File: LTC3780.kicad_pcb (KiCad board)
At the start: 2 copper layers, 100 x 60 mm, 62 parts, among them J1 Screw_Terminal_01x02, J2 Screw_Terminal_01x02, Q2 IPD100N04S402ATMA1, Q3 IPD100N04S402ATMA1, Q4 IPD100N04S402ATMA1, Q5 IPD100N04S402ATMA1, U1 LTC3780EGPBF

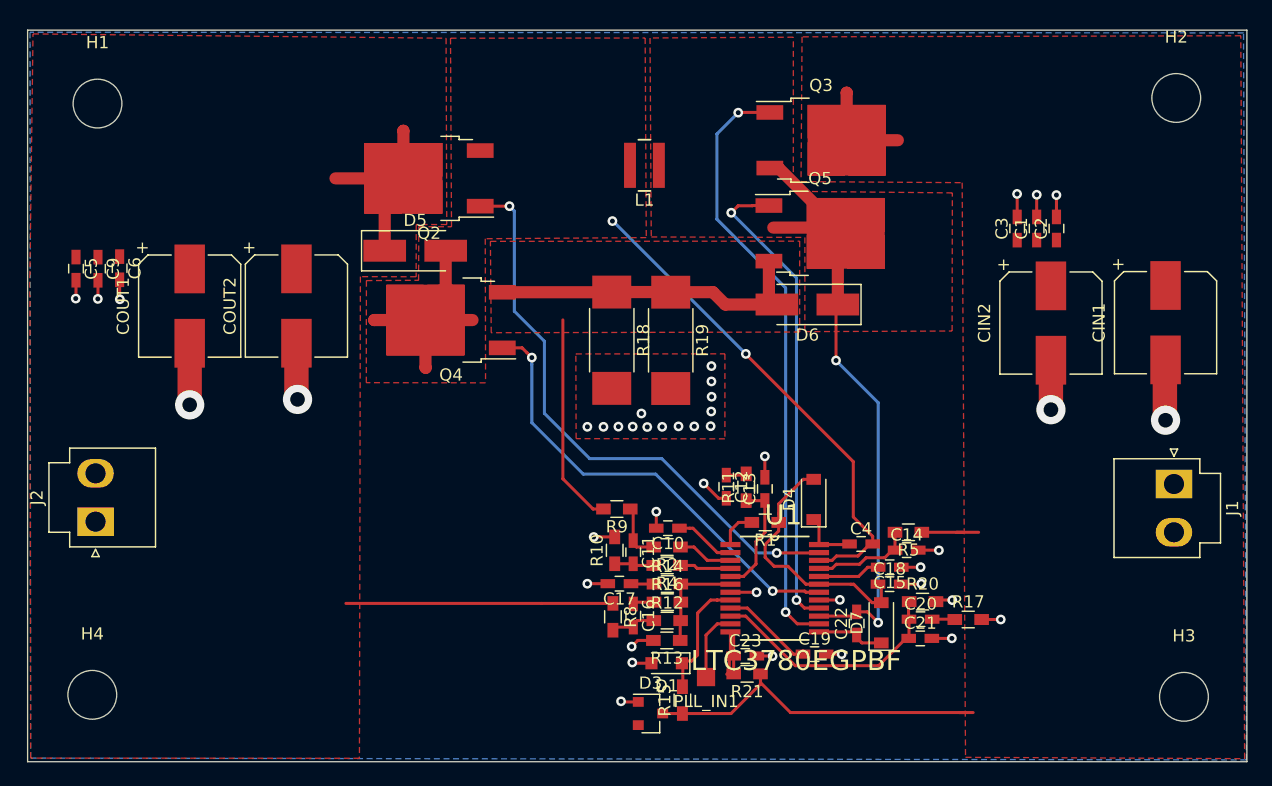
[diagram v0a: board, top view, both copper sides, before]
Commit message: Updating to latest version tidied routing
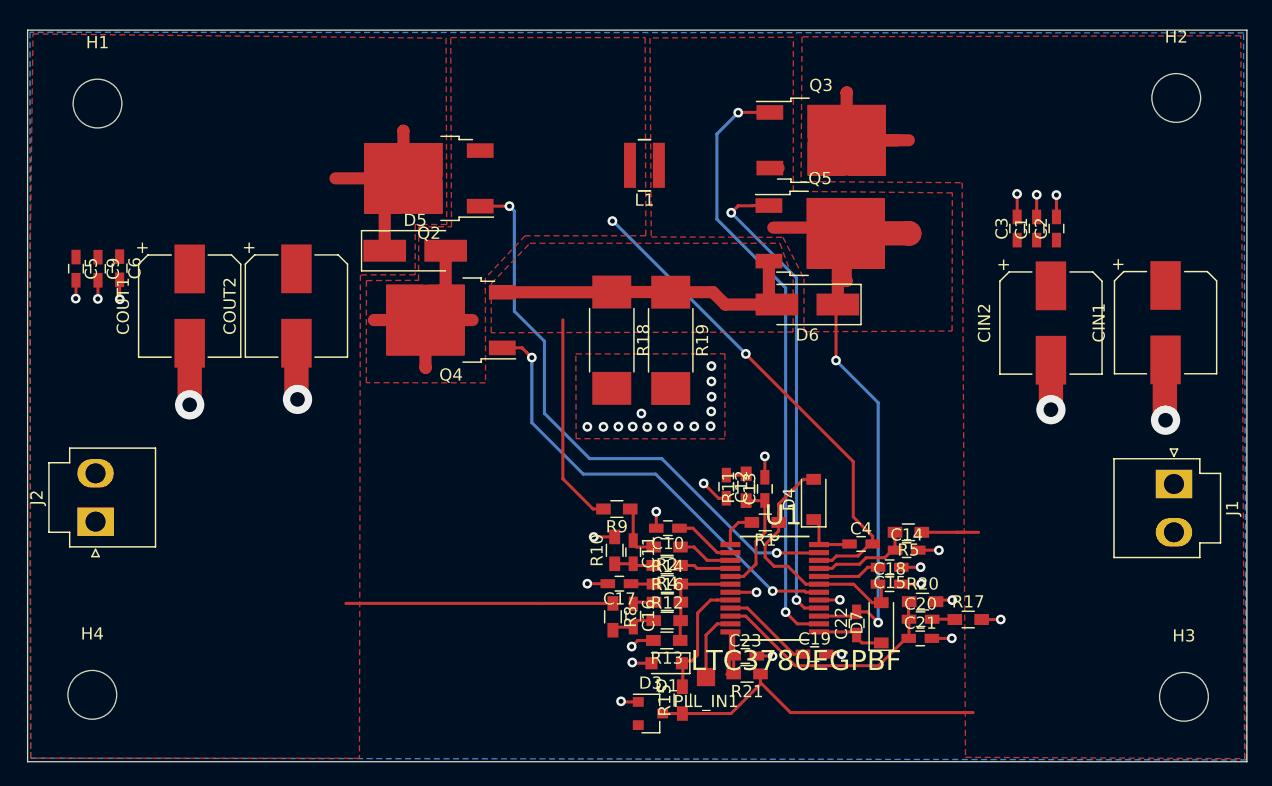
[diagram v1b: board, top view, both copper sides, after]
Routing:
- net +VSW: track 42.7 -> 47.9 mm
- net SW2: track 63.5 -> 60.4 mm
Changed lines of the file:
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@@
     (thickness 1.6)
     (drawings 6)
-    (tracks 348)
+    (tracks 355)
     (zones 0)
     (modules 62)
@@
   (segment (start 180.56606 102.98176) (end 194.41668 102.98176) (width 0.25) (layer F.Cu) (net 1))
   (segment (start 194.41668 102.98176) (end 194.88912 102.98176) (width 0.25) (layer F.Cu) (net 1))
+  (segment (start 185.17304 56.0451) (end 190.27648 56.0451) (width 1) (layer F.Cu) (net 1))
+  (segment (start 185.17304 52.1451) (end 185.2041 52.11404) (width 1) (layer F.Cu) (net 1))
   (via (at 211.328 79.0067) (size 2.4) (drill 1.2) (layers F.Cu B.Cu) (net 2))
   (segment (start 211.27466 79.0829) (end 211.27466 74.55608) (width 2) (layer F.Cu) (net 2) (status 10))
@@
   (segment (start 184.3024 74.10704) (end 184.3024 69.66712) (width 0.25) (layer F.Cu) (net 21) (status 20))
   (segment (start 184.45226 66.23518) (end 183.42242 65.20534) (width 0.25) (layer F.Cu) (net 21) (status 30))
-  (segment (start 179.44218 58.3251) (end 184.79742 63.68034) (width 0.25) (layer F.Cu) (net 21) (status 30))
   (segment (start 184.79742 63.68034) (end 185.09742 63.68034) (width 0.25) (layer F.Cu) (net 21) (status 30))
   (segment (start 178.87304 58.3251) (end 179.44218 58.3251) (width 0.25) (layer F.Cu) (net 21) (status 30))
   (segment (start 184.45226 64.3255) (end 185.09742 63.68034) (width 2.5) (layer F.Cu) (net 21))
-  (segment (start 179.59218 58.3251) (end 183.42242 62.15534) (width 1) (layer F.Cu) (net 21))
   (segment (start 178.87304 58.3251) (end 179.59218 58.3251) (width 1) (layer F.Cu) (net 21))
   (segment (start 184.45226 63.18518) (end 183.42242 62.15534) (width 1) (layer F.Cu) (net 21))
-  (segment (start 184.45226 69.51726) (end 184.45226 63.18518) (width 1) (layer F.Cu) (net 21))
   (segment (start 184.79742 63.68034) (end 184.32752 63.21044) (width 1) (layer F.Cu) (net 21))
   (segment (start 184.32752 63.21044) (end 179.15636 63.21044) (width 1) (layer F.Cu) (net 21))
+  (segment (start 190.29742 63.68034) (end 190.32028 63.7032) (width 2) (layer F.Cu) (net 21))
+  (segment (start 185.09742 63.68034) (end 190.29742 63.68034) (width 2) (layer F.Cu) (net 21))
+  (segment (start 184.45226 67.54622) (end 184.45226 63.18518) (width 1) (layer F.Cu) (net 21))
+  (segment (start 184.45226 69.51726) (end 184.45226 67.54622) (width 1) (layer F.Cu) (net 21))
+  (segment (start 185.16854 67.5767) (end 184.48274 67.5767) (width 1) (layer F.Cu) (net 21))
+  (segment (start 185.09742 67.50558) (end 185.16854 67.5767) (width 1) (layer F.Cu) (net 21))
+  (segment (start 184.48274 67.5767) (end 184.45226 67.54622) (width 1) (layer F.Cu) (net 21))
+  (segment (start 185.09742 63.68034) (end 185.09742 67.50558) (width 1) (layer F.Cu) (net 21))
   (segment (start 175.641 98.20652) (end 175.54952 98.298) (width 0.25) (layer F.Cu) (net 22) (status 30))
   (segment (start 175.641 96.3676) (end 175.641 98.20652) (width 0.25) (layer F.Cu) (net 22) (status 30))
@@
     (polygon
       (pts
-        (xy 180.80228 47.59452) (xy 169.04716 47.65802) (xy 169.14876 63.97752) (xy 181.7497 64.01308) (xy 181.74462 71.7423)
-        (xy 193.82232 71.6915) (xy 193.84264 60.3631) (xy 180.7972 60.23356)
+        (xy 180.80228 47.59452) (xy 169.04716 47.65802) (xy 169.14876 63.97752) (xy 179.95392 64.008) (xy 181.67604 67.39382)
+        (xy 181.67858 71.75246) (xy 193.82232 71.6915) (xy 193.84264 60.3631) (xy 180.7972 60.23356)
       )
     )
@@
     (polygon
       (pts
-        (xy 118.44274 47.32528) (xy 152.32126 47.67834) (xy 152.37714 62.95898) (xy 149.8727 62.95898) (xy 149.86762 67.24142)
-        (xy 145.29308 67.23126) (xy 145.21434 106.73334) (xy 118.2497 106.7181) (xy 118.1862 67.25158)
+        (xy 118.44274 47.32528) (xy 152.32126 47.67834) (xy 152.37714 62.95898) (xy 149.79142 62.9539) (xy 149.78126 67.0814)
+        (xy 145.29308 67.09156) (xy 145.21434 106.73334) (xy 118.2497 106.7181) (xy 118.1862 67.25158)
       )
     )
@@
     (polygon
       (pts
-        (xy 152.68448 47.67834) (xy 168.64838 47.65802) (xy 168.73982 64.03086) (xy 155.53436 64.1223) (xy 155.55976 75.94092)
-        (xy 145.77822 75.92822) (xy 145.78584 67.55638) (xy 150.06574 67.53098) (xy 150.08352 63.13424) (xy 152.76576 63.14186)
+        (xy 152.70226 47.625) (xy 168.64838 47.625) (xy 168.70426 63.881) (xy 158.79826 63.881) (xy 155.53944 67.35572)
+        (xy 155.55976 75.94092) (xy 145.77822 75.92822) (xy 145.78584 67.55638) (xy 150.0632 67.53352) (xy 150.08352 63.14186)
+        (xy 152.76576 63.1444)
       )
     )
@@
     (polygon
       (pts
-        (xy 155.956 64.3382) (xy 181.32298 64.32042) (xy 181.3179 71.77532) (xy 156.02458 71.8312)
+        (xy 156.0322 67.80022) (xy 159.19196 64.49314) (xy 179.705 64.49568) (xy 180.78704 67.4878) (xy 180.78196 71.77532)
+        (xy 156.02458 71.8312)
       )
     )
